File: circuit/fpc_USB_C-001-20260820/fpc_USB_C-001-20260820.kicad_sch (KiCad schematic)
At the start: 2 parts, among them P1 USB_C_Plug, P2 USB_C_Plug

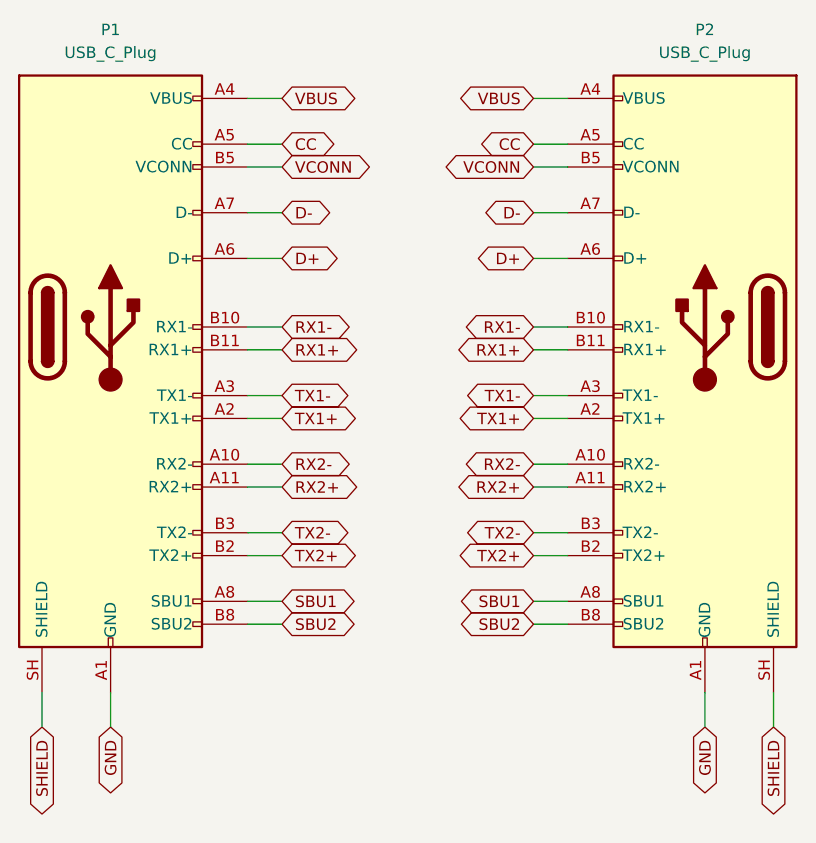
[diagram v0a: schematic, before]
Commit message: Update カメラ用のUSB-CのFPCケーブルを作ろうとした
フットプリントどうしよ
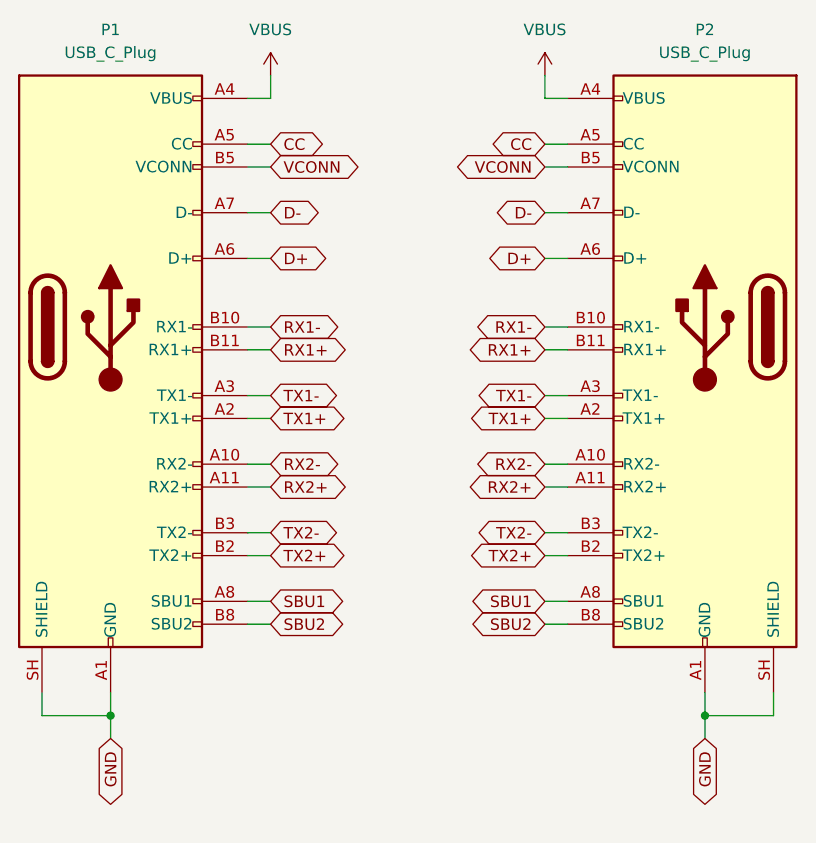
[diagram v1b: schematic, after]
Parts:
- P1, P2: footprint Connector_USB:USB_C_Receptacle_GCT_USB4105-xx-A_16P_TopMnt_Horizontal -> Connector_USB:USB_C_Plug_JAE_DX07P024AJ1
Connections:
- net SHIELD is gone; now on net GND: P1.SH (SHIELD), P2.SH (SHIELD)
